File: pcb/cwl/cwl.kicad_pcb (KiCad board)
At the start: 2 copper layers, 66.1 x 35 mm, 30 parts, among them J1 UEXT, J2 OpenTherm, J3 OLED_SH1106, J4 EXT_GPIO, J5 AUX, Q1 2N7002, SW1 EC12E24204A9, U1 LTV-817S-B, U2 LTV-817S-B

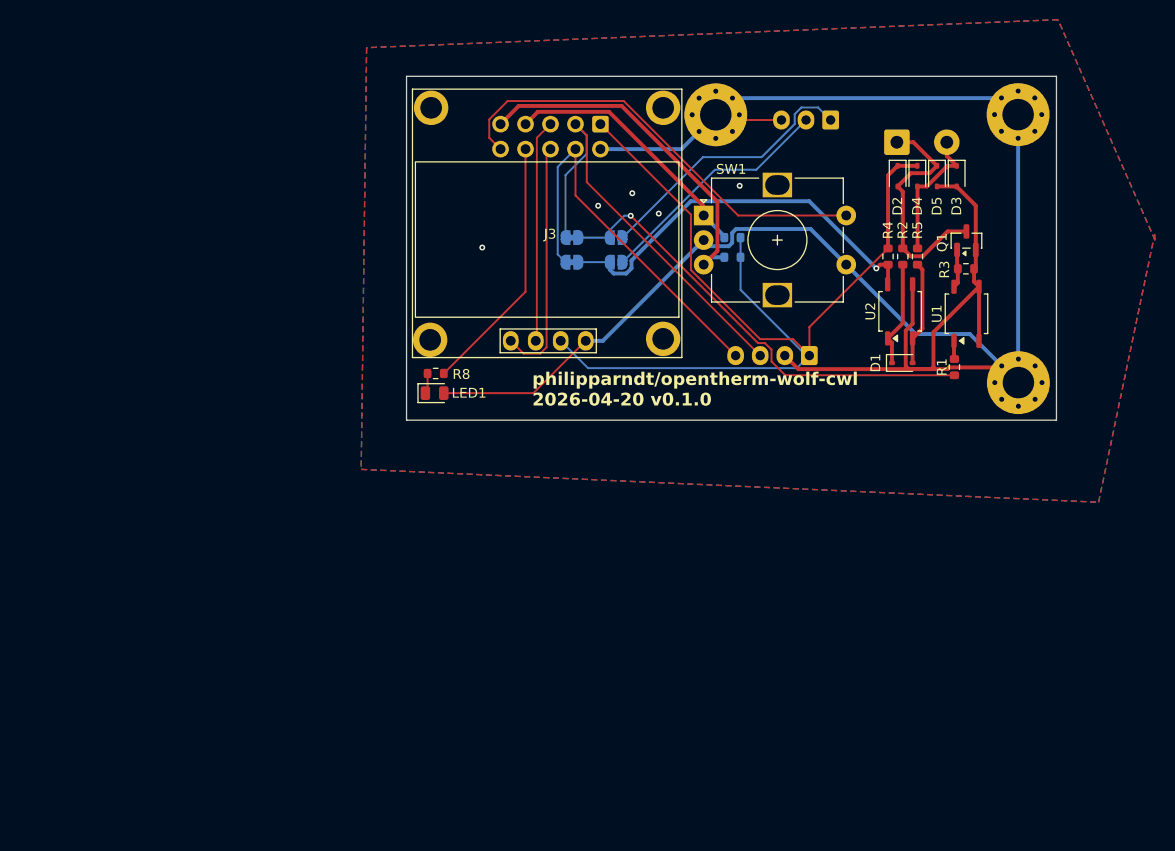
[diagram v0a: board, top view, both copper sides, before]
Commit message: new pcb
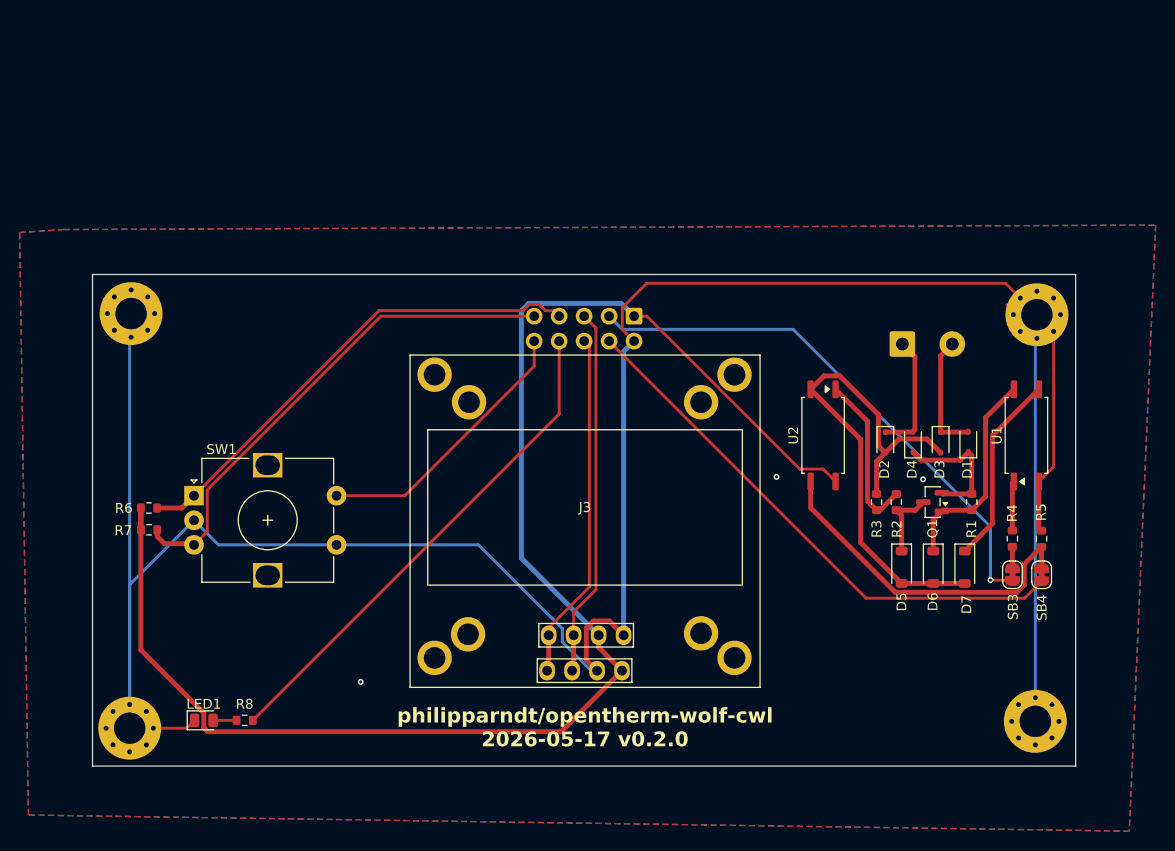
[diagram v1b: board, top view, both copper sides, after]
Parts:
- removed J4: EXT_GPIO, Connector_JST:JST_XH_B3B-XH-A_1x03_P2.50mm_Vertical
- removed J5: AUX, Connector_JST:JST_XH_B4B-XH-A_1x04_P2.50mm_Vertical
- removed SB1: GPIO4→OT_TX, Jumper:SolderJumper-2_P1.3mm_Open_RoundedPad1.0x1.5mm
- removed SB2: GPIO36→OT_RX, Jumper:SolderJumper-2_P1.3mm_Open_RoundedPad1.0x1.5mm
- added D6: BZT52C15, Diode_SMD:D_SOD-123, F.Cu at (125.3, 90.0)
- added D7: BZT52C4V3, Diode_SMD:D_SOD-123, F.Cu at (128.6, 90.0)
- added MH3: M3, MountingHole:MountingHole_3.2mm_M3_Pad_Via, F.Cu at (43.6, 106.4)
- D1: value BZX384-C4V7 -> 1N4148WS
- D5: value 1N4148WS -> BZT52C4V7; footprint Diode_SMD:D_SOD-323 -> Diode_SMD:D_SOD-123
- J3: value OLED_SH1106 -> OLED; footprint SSD1306:128x64OLED-MountingHoles -> SSD1306:128x64OLED-MountingHoles-Combined
- Q1: value 2N7002 -> BC858A
- R2: value 680 -> 220
- R3: value 4.7k -> 100
- R4: value 10k -> 330
- R5: value 1k -> 1.5k
- R6, R7, SB3, SB4: moved to F.Cu
- U1, U2: value LTV-817S-B -> PC817; footprint Package_SO:SOP-4_3.8x4.1mm_P2.54mm -> Package_SO:SOP-4_7.5x4.1mm_P2.54mm
- moved MH1 92.5 mm to (43.8, 64.2)
- moved MH4 69.7 mm to (135.7, 105.7)
- moved R7 65.5 mm to (45.6, 86.2), turned to 180 degrees
- moved R6 65.4 mm to (45.6, 84.0)
- moved SW1 59.2 mm to (50.2, 82.8)
- moved SB4 57.4 mm to (136.4, 90.8), turned to 90 degrees
- moved SB3 56.4 mm to (133.4, 90.8), turned to 90 degrees
- moved LED1 40.7 mm to (51.2, 105.6)
- moved R8 40.3 mm to (55.3, 105.6)
- moved D5 39.9 mm to (122.1, 90.0)
- moved R4 31.4 mm to (133.4, 87.1), turned to -90 degrees
- moved R5 31.4 mm to (136.4, 87.1)
- moved J3 27.6 mm to (72.1, 68.4), turned to 0 degrees
- moved D4 27.3 mm to (120.5, 77.3)
- moved D3 27.1 mm to (126.1, 77.3)
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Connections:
- D1 pad 1: RX_ANODE -> Net-(D1-K)
- D1 pad 2: RX_CATHODE -> OT+
- D2 pad 1: +3V3 -> Net-(D1-K)
- D2 pad 2: OT+ -> OT-
- D3 pad 1: OT- -> OT+
- D3 pad 2: GND -> Net-(D3-A)
- D4 pad 1: +3V3 -> OT-
- D4 pad 2: OT- -> Net-(D3-A)
- D5 pad 1: OT+ -> Net-(D5-K)
- D5 pad 2: GND -> Net-(D3-A)
- J2 pad 1: OT+ -> OT-
- J2 pad 2: OT- -> OT+
- J3 pad 1: GND -> +3V3
- J3 pad 2: +3V3 -> GND
- LED1 pad 1: LED_ANODE -> GND
- LED1 pad 2: GND -> Net-(LED1-A)
- Q1 pad 1: TX_GATE -> Net-(D6-K)
- Q1 pad 2: GND -> Net-(D1-K)
- Q1 pad 3: OT+ -> Net-(D5-K)
- R1 pad 1: OT_TX_SIG -> Net-(D1-K)
- R1 pad 2: TX_LED -> Net-(D6-K)
- R2 pad 1: OT+ -> Net-(R2-Pad1)
- R2 pad 2: RX_ANODE -> Net-(D5-K)
- R3 pad 1: TX_GATE -> Net-(R2-Pad1)
- R3 pad 2: GND -> Net-(D3-A)
- R4 pad 1: OT_RX_SIG -> Net-(R4-Pad1)
- R4 pad 2: +3V3 -> OT_TX_SIG
- R5 pad 1: RX_CATHODE -> OT_RX_SIG
- R5 pad 2: OT- -> GND
- R6 pad 1: ENC_CLK -> +3V3
- R6 pad 2: +3V3 -> ENC_CLK
- R8 pad 2: LED_ANODE -> Net-(LED1-A)
- U1 pad 1: TX_LED -> Net-(R4-Pad1)
- U1 pad 3: GND -> Net-(D7-K)
- U1 pad 4: TX_GATE -> Net-(D6-K)
- U2 pad 1: RX_ANODE -> Net-(R2-Pad1)
- U2 pad 2: RX_CATHODE -> Net-(D3-A)
- U2 pad 3: GND -> OT_RX_SIG
- U2 pad 4: OT_RX_SIG -> +3V3
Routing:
- net GND: track 215.6 -> 272.3 mm, vias 5 -> 3
- net Net-(D3-A): track 0.00 -> 54.6 mm
- net +3V3: track 101.4 -> 153.1 mm
- net OT_TX_SIG: track 47.0 -> 2.19 mm, vias 1 -> 0
- net GPIO4: track 27.8 -> 0.00 mm
- net LED_GPIO: track 26.3 -> 51.5 mm
- net GPIO36: track 24.6 -> 0.00 mm
- net ENC_CLK: track 27.5 -> 50.0 mm
- net Net-(D6-K): track 0.00 -> 21.6 mm
- net Net-(D7-K): track 0.00 -> 19.6 mm
- net ENC_SW: track 45.4 -> 28.1 mm
- net Net-(R2-Pad1): track 0.00 -> 16.7 mm
- net ENC_DT: track 36.3 -> 51.5 mm
- net UEXT_RXD: track 40.3 -> 55.5 mm
- net SCL: track 22.7 -> 37.6 mm
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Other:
- board size 66.1 x 35 mm -> 100 x 50 mm
- board text added: "philipparndt/opentherm-wolf-cwl 2026-05-17 v0.2.0"
- board text removed: "Configure"
- board text removed: "J4"
- board text removed: "J4 (EXT_GPIO) 1: GPIO4 (OT TX) 2: GPIO36 (OT RX) 3: GND"
- board text removed: "J5 (AUX) 1: +3V3 2: GND 3: TXD 4: RXD"
- board text removed: "UEXT"
- board text removed: "philipparndt/opentherm-wolf-cwl 2026-04-20 v0.1.0"
